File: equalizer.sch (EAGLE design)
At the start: 34 parts

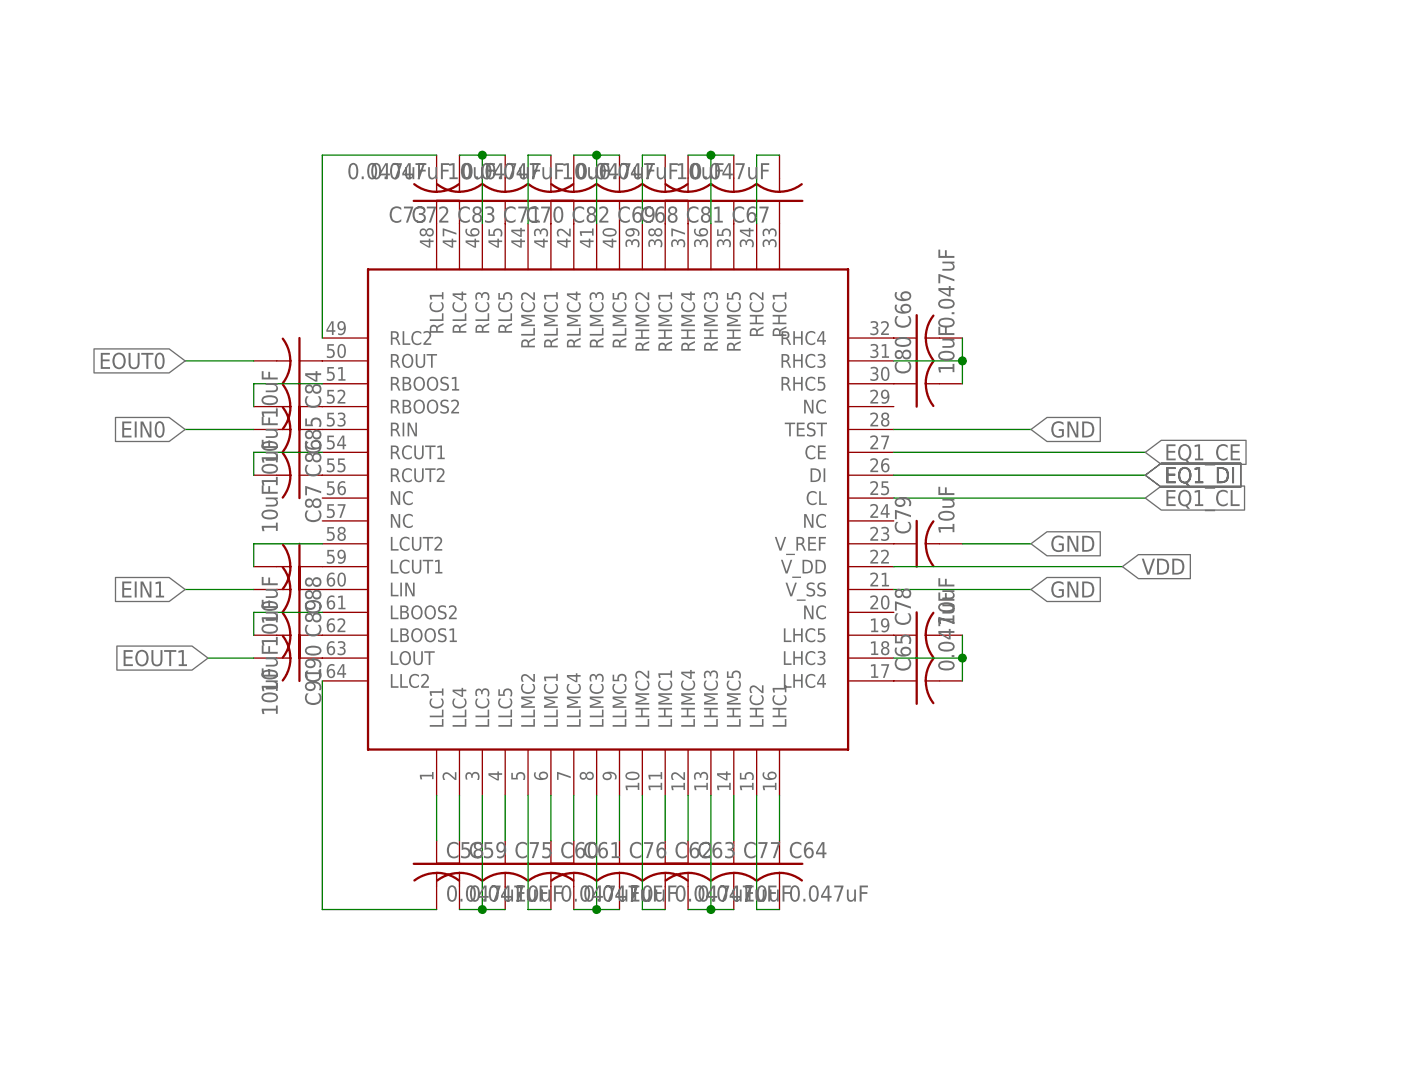
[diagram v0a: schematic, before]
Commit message: corrections
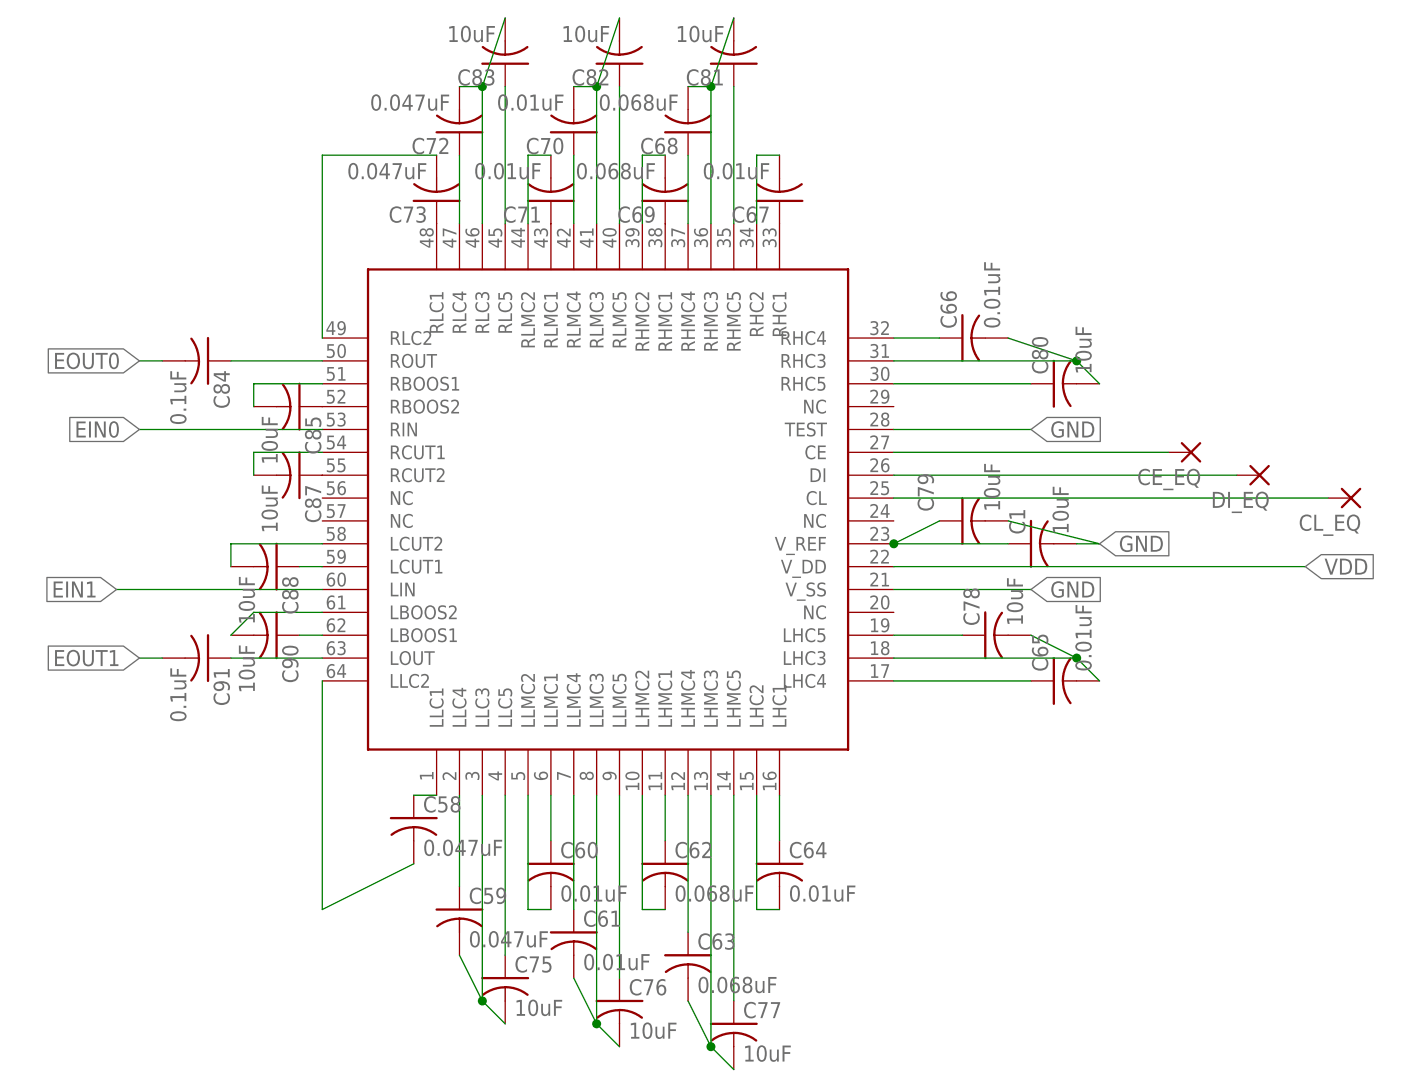
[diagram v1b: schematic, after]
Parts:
- removed C86, C89: 10uF, rcl:C-USC0402
- added C1: 10uF, rcl:C-USC0402
- added CE_EQ, CL_EQ, DI_EQ: (no value), wirepad:SMD2
- C60, C61, C64, C65, C66, C67, C70, C71: value 0.047uF -> 0.01uF
- C62, C63, C68, C69: value 0.047uF -> 0.068uF
- C84, C91: value 10uF -> 0.1uF
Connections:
- removed net N$199: C86.1, U$14.RIN
- removed net N$202: C89.1, U$14.LIN
- net EIN0: now also U$14.RIN; no longer C86.2
- net EIN1: now also U$14.LIN; no longer C89.2
- net EQ1_CE: now also CE_EQ.P
- net EQ1_CL: now also CL_EQ.P
- net EQ1_DI: now also DI_EQ.P
- net GND: now also C1.2
- net N$192: now also C1.1
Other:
- moved on the sheet: C58, C59, C61, C63, C65, C66, C68, C70, C72, C75, C76, C77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
